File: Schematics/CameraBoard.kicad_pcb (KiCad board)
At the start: 4 copper layers, 50 x 100 mm, 74 parts, among them J1 Microsemi_FlashPro-JTAG-10, J3 USB_C_Receptacle_USB2.0_16P, U1 STM32F405RGT6, U2 LDL1117-3.3, U3 TPS22917DBVR, U4 SN65HVD230, U5 TPS22917DBVR, U6 TPS22917DBVR, Y1 8mhz

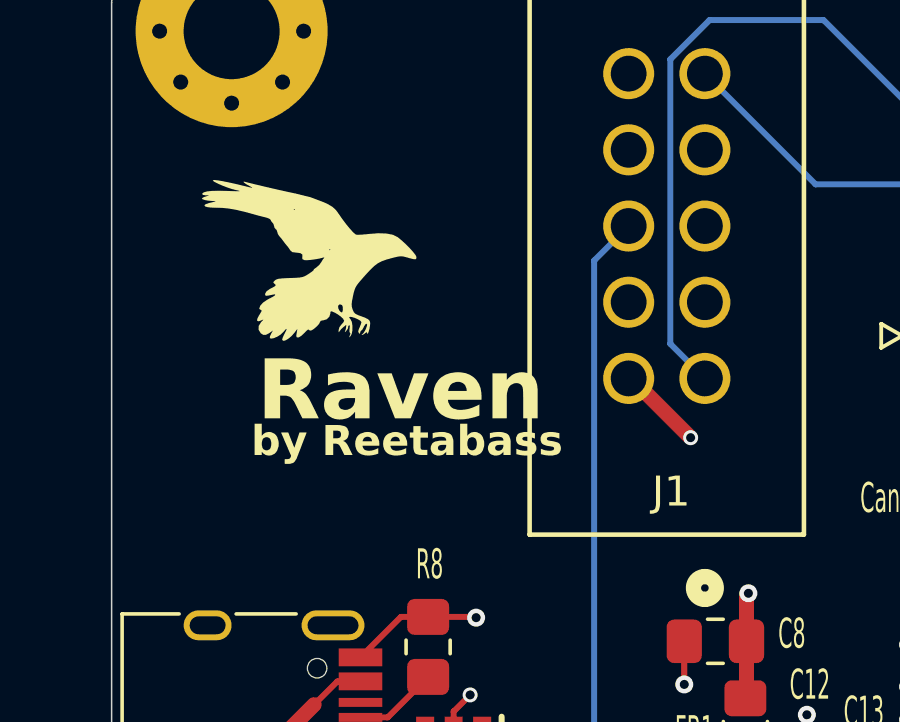
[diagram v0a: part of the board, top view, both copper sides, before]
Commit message: output files completed quote obtained
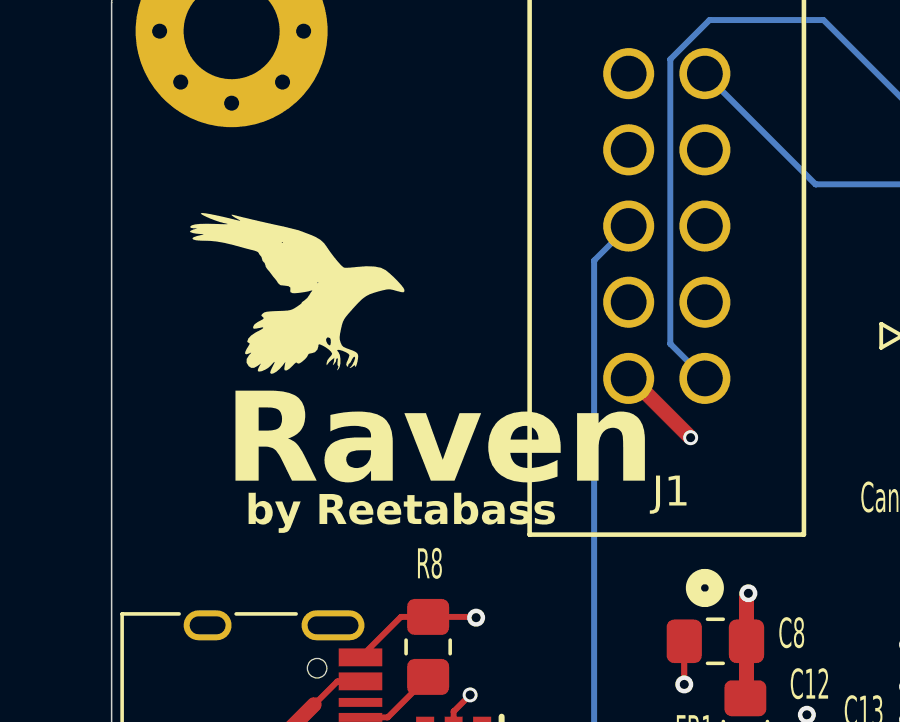
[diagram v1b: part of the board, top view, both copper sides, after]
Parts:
- moved G*** 1.17 mm to (78.4, 52.7)
